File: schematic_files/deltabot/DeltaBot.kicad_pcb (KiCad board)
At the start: 2 copper layers, 177.6 x 100 mm, 23 parts, among them J1 USB C PD Modulle, J3 MOTOR_L, J4 MOTOR_R, J5 C1_LIDAR, SW1 SW_SPDT, U1 Radxa_ROCK5B, U2 Buck Converter

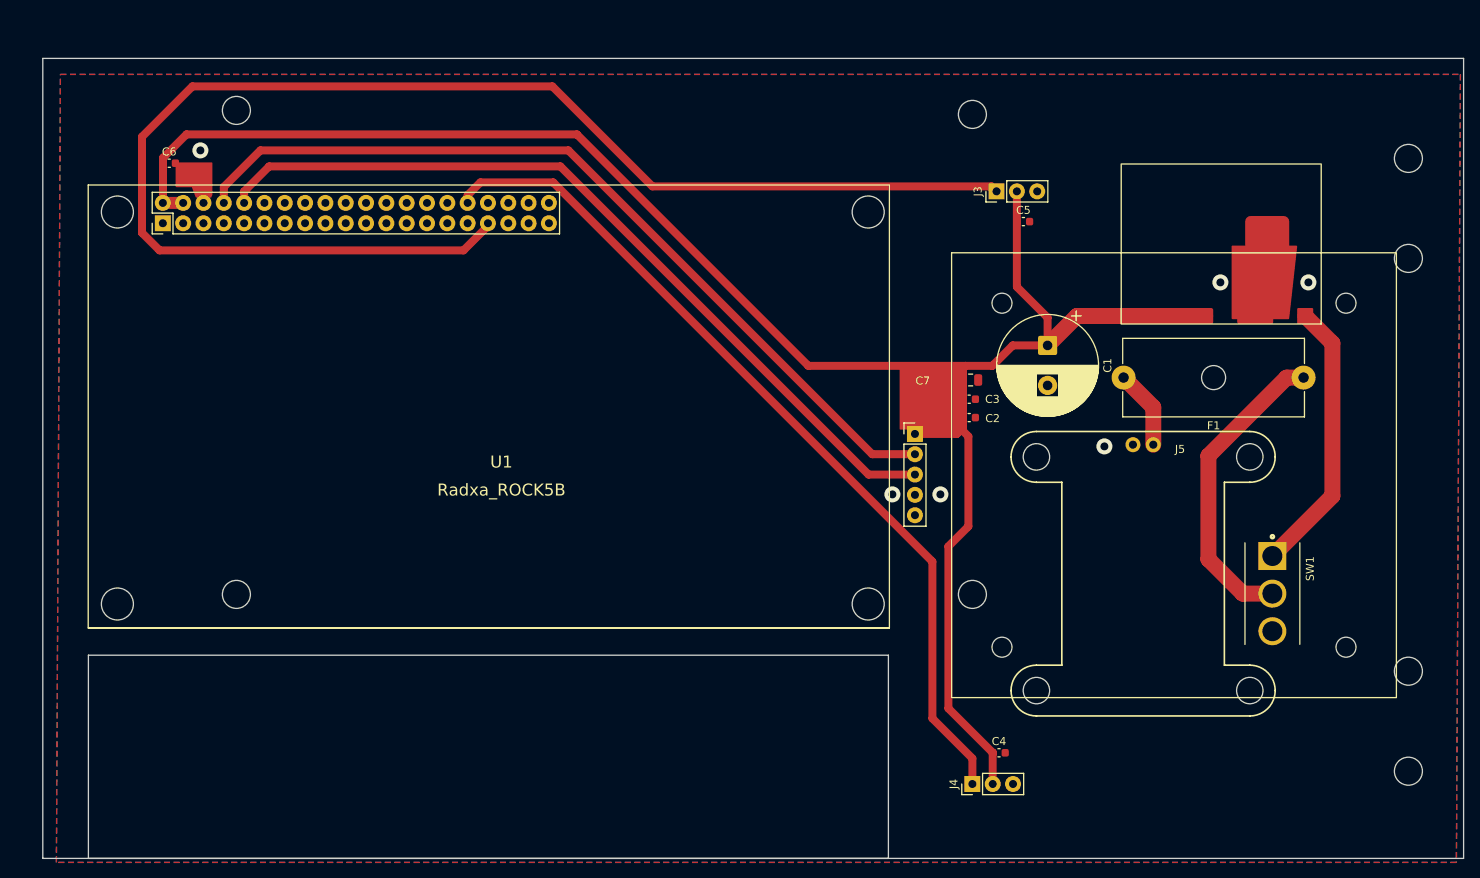
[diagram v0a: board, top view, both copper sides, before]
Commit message: pcb v2
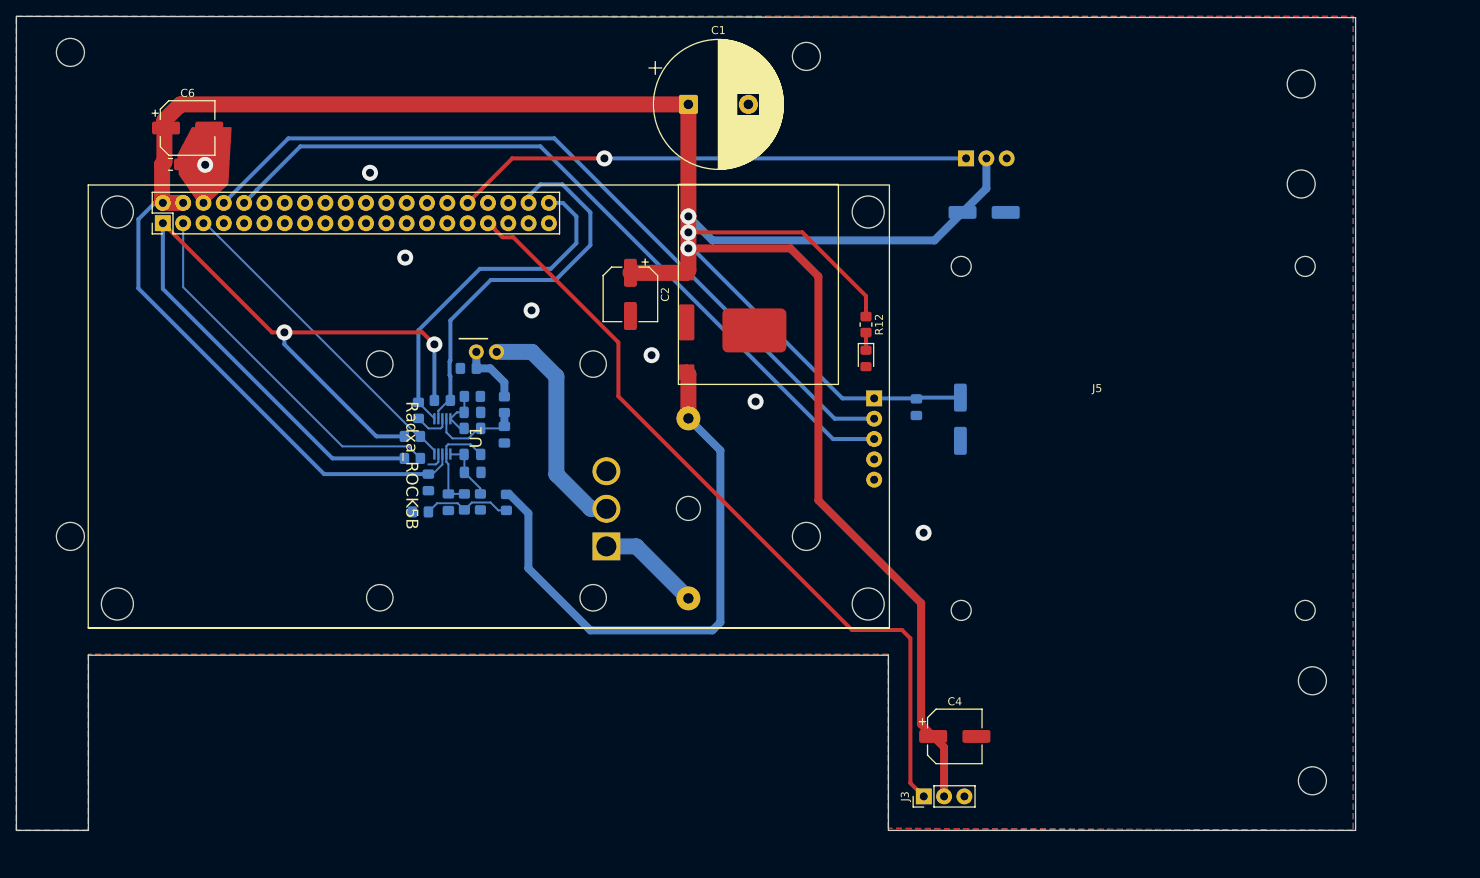
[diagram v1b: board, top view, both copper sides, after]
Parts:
- added C10: 10nF, Capacitor_SMD:C_0805_2012Metric_Pad1.18x1.45mm_HandSolder, B.Cu at (90.0, 97.8)
- added C11: 10nF, Capacitor_SMD:C_0805_2012Metric_Pad1.18x1.45mm_HandSolder, B.Cu at (90.0, 105.2)
- added C12: 100nF, Capacitor_SMD:C_0805_2012Metric_Pad1.18x1.45mm_HandSolder, B.Cu at (84.5, 106.5)
- added C13: 10nF, Capacitor_SMD:C_0805_2012Metric_Pad1.18x1.45mm_HandSolder, B.Cu at (87.0, 109.0)
- added C14: 100nF, Capacitor_SMD:C_0805_2012Metric_Pad1.18x1.45mm_HandSolder, B.Cu at (90.0, 99.8)
- added C15: 100nF, Capacitor_SMD:C_0805_2012Metric_Pad1.18x1.45mm_HandSolder, B.Cu at (90.0, 103.0)
- added C8: 100nF, Capacitor_SMD:C_0805_2012Metric_Pad1.18x1.45mm_HandSolder, F.Cu at (52.2, 66.8)
- added C9: 10nF, Capacitor_SMD:C_0805_2012Metric_Pad1.18x1.45mm_HandSolder, B.Cu at (94.0, 100.5)
- added D1: LED, LED_SMD:LED_0805_2012Metric_Pad1.15x1.40mm_HandSolder, F.Cu at (139.2, 91.0)
- added IC1: ADS1115LIDGSR, deltabot:SOP50P490X110-10N, B.Cu at (86.2, 100.8)
- added R1: 10R, Resistor_SMD:R_0805_2012Metric_Pad1.20x1.40mm_HandSolder, B.Cu at (91.0, 108.9)
- added R10: 10k, Resistor_SMD:R_0805_2012Metric_Pad1.20x1.40mm_HandSolder, B.Cu at (94.2, 109.0)
- added R11: 4k7, Resistor_SMD:R_0805_2012Metric_Pad1.20x1.40mm_HandSolder, B.Cu at (83.5, 110.2)
- added R12: 1k, Resistor_SMD:R_0805_2012Metric_Pad1.20x1.40mm_HandSolder, F.Cu at (139.2, 86.8)
- added R2: 10R, Resistor_SMD:R_0805_2012Metric_Pad1.20x1.40mm_HandSolder, B.Cu at (94.0, 96.8)
- added R3: 10R, Resistor_SMD:R_0805_2012Metric_Pad1.20x1.40mm_HandSolder, B.Cu at (90.0, 95.8)
- added R4: 10k, Resistor_SMD:R_0805_2012Metric_Pad1.20x1.40mm_HandSolder, B.Cu at (83.2, 97.5)
- added R5: 10R, Resistor_SMD:R_0805_2012Metric_Pad1.20x1.40mm_HandSolder, B.Cu at (89.0, 108.9)
- added R6: 10k, Resistor_SMD:R_0805_2012Metric_Pad1.20x1.40mm_HandSolder, B.Cu at (86.2, 96.2)
- added R7: 10k, Resistor_SMD:R_0805_2012Metric_Pad1.20x1.40mm_HandSolder, B.Cu at (82.5, 100.8)
- added R8: 10k, Resistor_SMD:R_0805_2012Metric_Pad1.20x1.40mm_HandSolder, B.Cu at (82.5, 103.5)
- added R9: shunt resistor (wire), Resistor_SMD:R_0805_2012Metric_Pad1.20x1.40mm_HandSolder, B.Cu at (89.5, 92.2)
- C1: footprint Capacitor_THT:CP_Radial_D12.5mm_P5.00mm -> Capacitor_THT:CP_Radial_D16.0mm_P7.50mm
- C2: footprint Capacitor_SMD:C_0603_1608Metric -> Capacitor_SMD:CP_Elec_6.3x3
- C3: value 0.1uF -> 100nF; footprint Capacitor_SMD:C_0603_1608Metric -> Capacitor_SMD:C_0805_2012Metric_Pad1.18x1.45mm_HandSolder; moved to B.Cu
- C4: value 1uF -> 220uF; footprint Capacitor_SMD:C_0603_1608Metric -> Capacitor_SMD:CP_Elec_6.3x3
- C5: value 1uF -> 220uF; footprint Capacitor_SMD:C_0603_1608Metric -> Capacitor_SMD:CP_Elec_6.3x3; moved to B.Cu
- C6: value 1uF -> 10uF; footprint Capacitor_SMD:C_0603_1608Metric -> Capacitor_SMD:CP_Elec_6.3x3
- C7: value 5uF -> 4u7F; footprint Capacitor_SMD:C_0805_2012Metric -> Capacitor_SMD:CP_Elec_6.3x3; moved to B.Cu
- F1, J1, J4, J5, SW1: moved to B.Cu
- moved SW1 83.9 mm to (106.8, 109.8), turned to 90 degrees
- moved U2 80.7 mm to (115.8, 94.2), turned to 90 degrees
- moved J4 78.2 mm to (151.7, 66.0), turned to -90 degrees
- moved F1 77.1 mm to (117.0, 98.5), turned to -90 degrees
- moved J3 76.2 mm to (146.4, 145.8)
- moved C1 54.1 mm to (117.0, 59.2), turned to 0 degrees
- moved J1 49.8 mm to (108.6, 124.3)
- moved C2 45.1 mm to (109.8, 83.0), turned to -90 degrees
- moved REF** 22.0 mm to (131.8, 113.2)
- moved REF** 22.0 mm to (131.8, 53.2)
- moved REF** 22.0 mm to (39.8, 113.2)
- moved REF** 22.0 mm to (39.8, 52.8)
- moved REF** 16.3 mm to (193.6, 69.2)
- moved REF** 16.3 mm to (193.6, 56.7)
- moved REF** 12.1 mm to (195.0, 143.8)
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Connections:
- F1 pad 1: Net-(SW1-B) -> +9V
- F1 pad 2: Net-(J1-VCC) -> Net-(SW1-A)
- J1 pad 2: GND -> shunt
- SW1 pad 1: +9V -> Net-(SW1-A)
- SW1 pad 2: Net-(SW1-B) -> Net-(J1-VCC)
- U1 pad 1: unconnected-(U1-3.3V-Pad1) -> +3.3V
- U1 pad 3: unconnected-(U1-I2C7_SDA-Pad3) -> SDA
- U1 pad 38: unconnected-(U1-GPIO4_A6-Pad38) -> ALERT
- U1 pad 40: unconnected-(U1-GPIO4_A7-Pad40) -> ADDR
- U1 pad 5: unconnected-(U1-I2C7_SCL-Pad5) -> SCL
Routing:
- net +5V: track 242.2 -> 374.2 mm, vias 0 -> 3
- net +3.3V: track 0.00 -> 115.7 mm, vias 0 -> 2
- net PWM_L: track 172.6 -> 99.1 mm
- net ALERT: track 0.00 -> 49.3 mm
- net SDA: track 0.00 -> 48.9 mm
- net PWM_R: track 109.2 -> 64.4 mm, vias 0 -> 1
- net ADDR: track 0.00 -> 43.6 mm
- net SCL: track 0.00 -> 41.1 mm
- net Net-(SW1-B): track 38.7 -> 0.00 mm
- net +9V: track 34.5 -> 71.3 mm
- net Net-(J1-VCC): track 9.92 -> 29.0 mm
- net Net-(IC1-AIN3): track 0.00 -> 13.0 mm
- net Net-(SW1-A): track 0.00 -> 12.9 mm
- net Net-(IC1-AIN0): track 0.00 -> 11.6 mm
- net Net-(R10-Pad2): track 0.00 -> 11.3 mm
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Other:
- board size 177.6 x 100 mm -> 167.4 x 101.8 mm
